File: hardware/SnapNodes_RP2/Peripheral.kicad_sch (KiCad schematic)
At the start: 42 parts, among them J10 LCD, J11 USB_C, SW1 Center, SW2 Left, SW3 Bottom, SW4 Right, SW5 Top, U8 LSM6DS3, U9 AW9523B

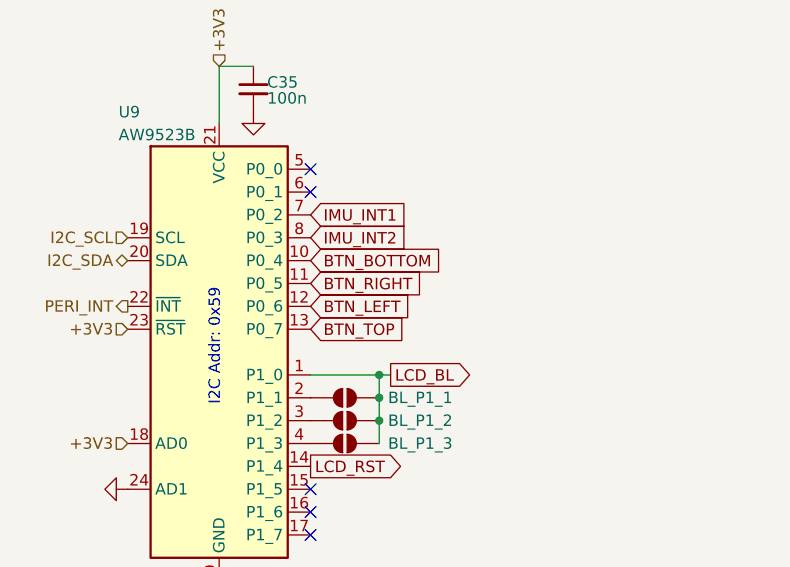
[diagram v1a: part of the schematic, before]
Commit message: PCB minor changes
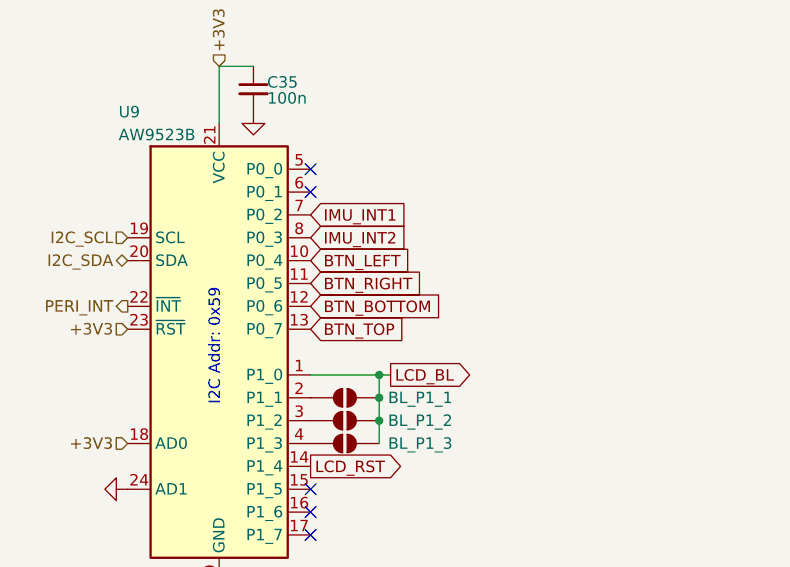
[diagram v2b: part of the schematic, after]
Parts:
- R31, R42, R43, R44, R45, R46, R47: Link https://www.lcsc.com/product-detail/C2907002.html -> https://www.lcsc.com/product-detail/C2906980.html
- R32, R33: Link https://www.lcsc.com/product-detail/C2907002.html -> https://www.lcsc.com/product-detail/C2907044.html
- SW1: Link (none) -> https://www.lcsc.com/product-detail/C2837550.html
- SW2, SW3, SW4, SW5: Link (none) -> https://www.lcsc.com/product-detail/C2837549.html
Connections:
- net BTN_BOTTOM: now also U9.12 (P0_6); no longer U9.10 (P0_4)
- net BTN_LEFT: now also U9.10 (P0_4); no longer U9.12 (P0_6)
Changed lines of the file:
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@@
 	(global_label "BTN_LEFT"
 		(shape input)
-		(at 49.53 48.26 0)
+		(at 49.53 43.18 0)
 		(fields_autoplaced yes)
 		(effects
@@
 		)
 		(property "Intersheetrefs" "${INTERSHEET_REFS}"
-			(at 61.2842 48.26 0)
+			(at 61.2842 43.18 0)
 			(effects
 				(font
@@
 	(global_label "BTN_BOTTOM"
 		(shape input)
-		(at 49.53 43.18 0)
+		(at 49.53 48.26 0)
 		(fields_autoplaced yes)
 		(effects
@@
 		)
 		(property "Intersheetrefs" "${INTERSHEET_REFS}"
-			(at 64.3685 43.18 0)
+			(at 64.3685 48.26 0)
 			(effects
 				(font
@@
 			)
 		)
-		(property "Link" "https://www.lcsc.com/product-detail/C2907002.html"
+		(property "Link" "https://www.lcsc.com/product-detail/C2906980.html"
 			(at 252.73 38.1 90)
 			(effects
@@
 			)
 		)
-		(property "Link" "https://www.lcsc.com/product-detail/C2907002.html"
+		(property "Link" "https://www.lcsc.com/product-detail/C2907044.html"
 			(at 59.69 129.54 90)
 			(effects
@@
 			)
 		)
+		(property "Link" "https://www.lcsc.com/product-detail/C2837550.html"
+			(at 153.67 156.21 0)
+			(effects
+				(font
+					(size 1.27 1.27)
+				)
+				(hide yes)
+			)
+		)
 		(pin "1"
 		)
@@
 			)
 		)
-		(property "Link" "https://www.lcsc.com/product-detail/C2907002.html"
+		(property "Link" "https://www.lcsc.com/product-detail/C2906980.html"
 			(at 250.19 38.1 90)
 			(effects
@@
 			)
 		)
+		(property "Link" "https://www.lcsc.com/product-detail/C2837549.html"
+			(at 153.67 129.54 0)
+			(effects
+				(font
+					(size 1.27 1.27)
+				)
+				(hide yes)
+			)
+		)
 		(pin "1"
 		)
@@
 			)
 		)
-		(property "Link" "https://www.lcsc.com/product-detail/C2907002.html"
+		(property "Link" "https://www.lcsc.com/product-detail/C2906980.html"
 			(at 134.62 158.75 90)
 			(effects
@@
 			)
 		)
-		(property "Link" "https://www.lcsc.com/product-detail/C2907002.html"
+		(property "Link" "https://www.lcsc.com/product-detail/C2906980.html"
 			(at 134.62 123.19 90)
 			(effects
@@
 			)
 		)
+		(property "Link" "https://www.lcsc.com/product-detail/C2837549.html"
+			(at 153.67 147.32 0)
+			(effects
+				(font
+					(size 1.27 1.27)
+				)
+				(hide yes)
+			)
+		)
 		(pin "1"
 		)
@@
 			)
 		)
+		(property "Link" "https://www.lcsc.com/product-detail/C2837549.html"
+			(at 153.67 120.65 0)
+			(effects
+				(font
+					(size 1.27 1.27)
+				)
+				(hide yes)
+			)
+		)
 		(pin "1"
 		)
@@
 			)
 		)
-		(property "Link" "https://www.lcsc.com/product-detail/C2907002.html"
+		(property "Link" "https://www.lcsc.com/product-detail/C2906980.html"
 			(at 134.62 140.97 90)
 			(effects
@@
 			)
 		)
-		(property "Link" "https://www.lcsc.com/product-detail/C2907002.html"
+		(property "Link" "https://www.lcsc.com/product-detail/C2907044.html"
 			(at 59.69 132.08 90)
 			(effects
@@
 			)
 		)
+		(property "Link" "https://www.lcsc.com/product-detail/C2837549.html"
+			(at 153.67 138.43 0)
+			(effects
+				(font
+					(size 1.27 1.27)
+				)
+				(hide yes)
+			)
+		)
 		(pin "1"
 		)
@@
 			)
 		)
-		(property "Link" "https://www.lcsc.com/product-detail/C2907002.html"
+		(property "Link" "https://www.lcsc.com/product-detail/C2906980.html"
 			(at 134.62 132.08 90)
 			(effects
@@
 			)
 		)
-		(property "Link" "https://www.lcsc.com/product-detail/C2907002.html"
+		(property "Link" "https://www.lcsc.com/product-detail/C2906980.html"
 			(at 134.62 149.86 90)
 			(effects
